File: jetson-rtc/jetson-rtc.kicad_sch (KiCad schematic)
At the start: 11 parts, among them J1 Conn_01x04, J2 Conn_02x20_Odd_Even, SW1 SW_Push, U1 DS3231MZ

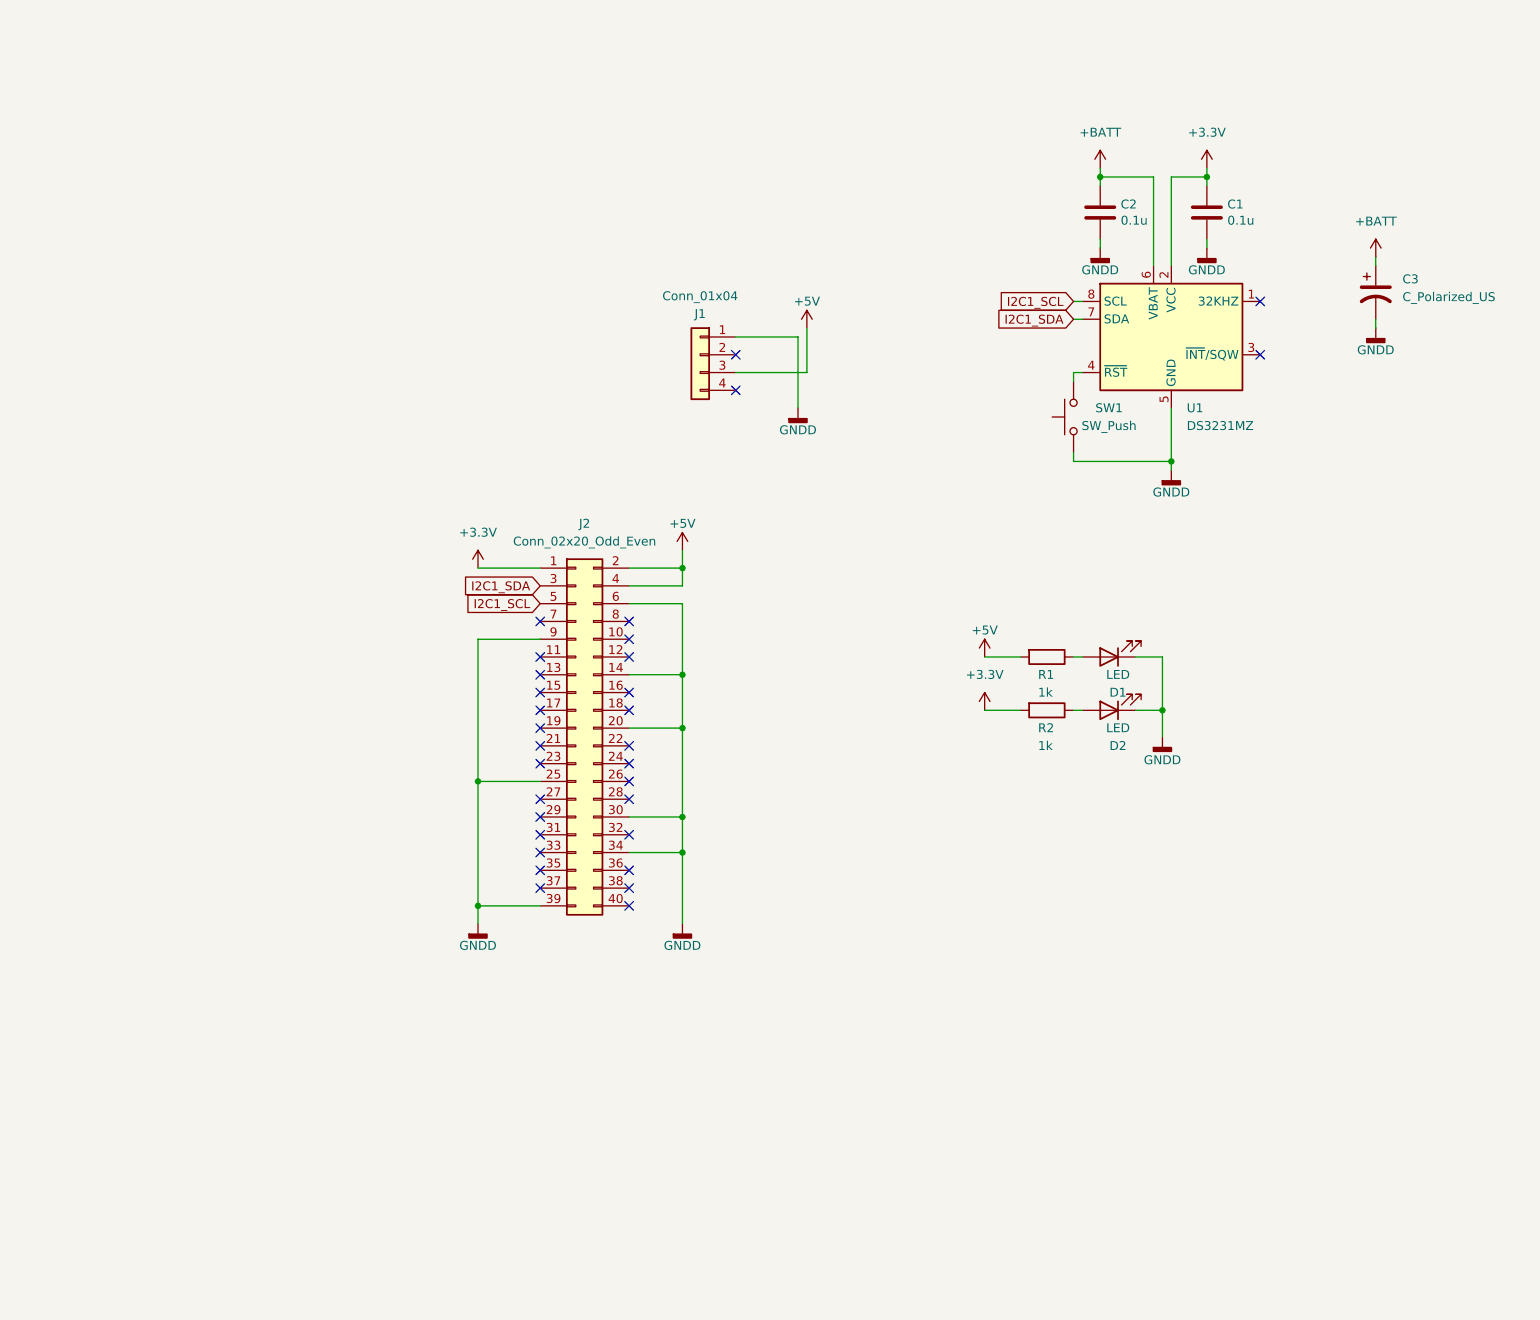
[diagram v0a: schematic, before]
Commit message: 回路図清掃
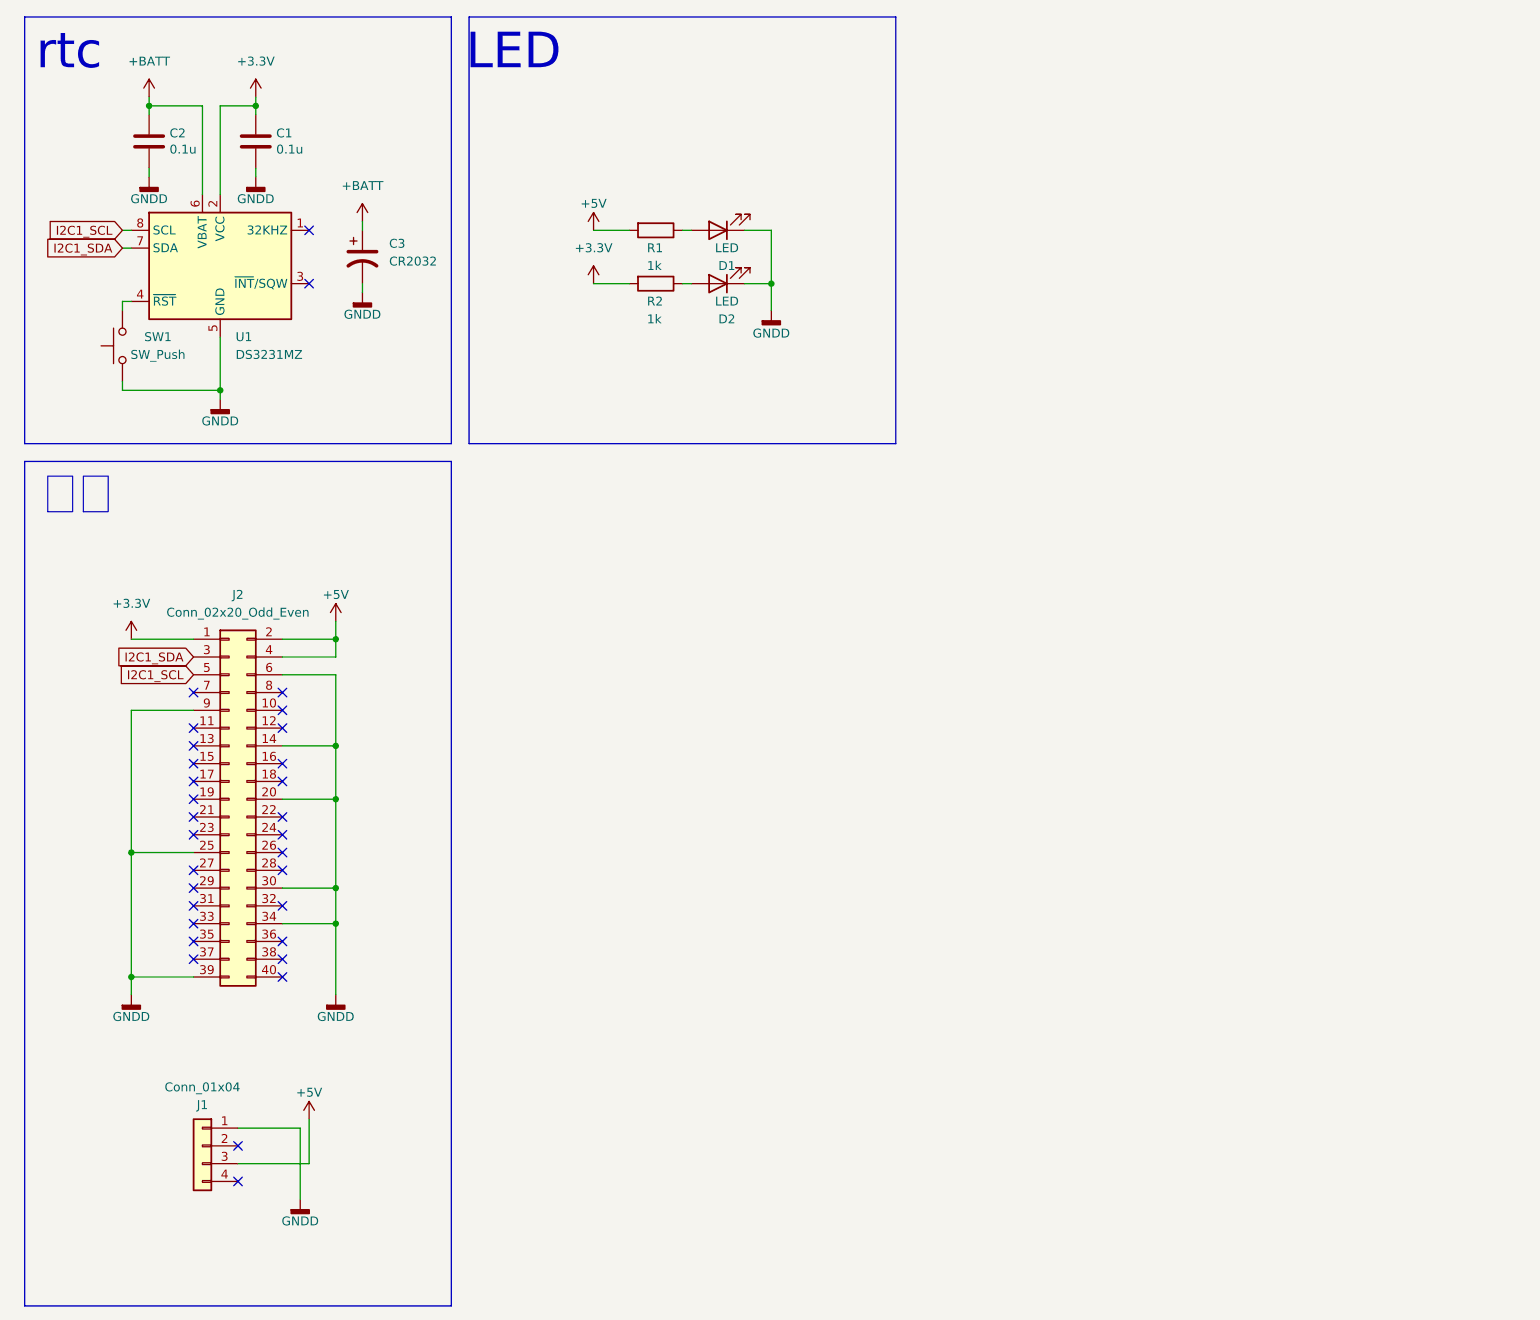
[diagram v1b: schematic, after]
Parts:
- C3: value C_Polarized_US -> CR2032
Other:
- note added: "LED"
- note added: "rtc"
- note added: "端子"
- moved on the sheet: C1, C2, C3, D1, D2, J1, J2, R1, R2, SW1, U1
